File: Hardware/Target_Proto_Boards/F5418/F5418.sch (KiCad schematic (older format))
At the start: 51 parts, among them J1 LED_P4.1, J10 PORT4, J11 PORT8, J12 JTAG/SBW, J13 VCC, J14 GND, J15 +5V, J16 GND, J17 VSEL, J18 LogAna, J19 AS, J2 PORT1, J3 PORT5, J4 DEBUG, J5 PORT2, J6 PORT6, J7 USB_B_Micro, J8 PORT3, J9 PORT7, SW1 RESET, SW2 TL-2203, U1 MSP430F5418IPNR, U2 HT7533-1, Y1 32768 12pF, Y2 25 MHz

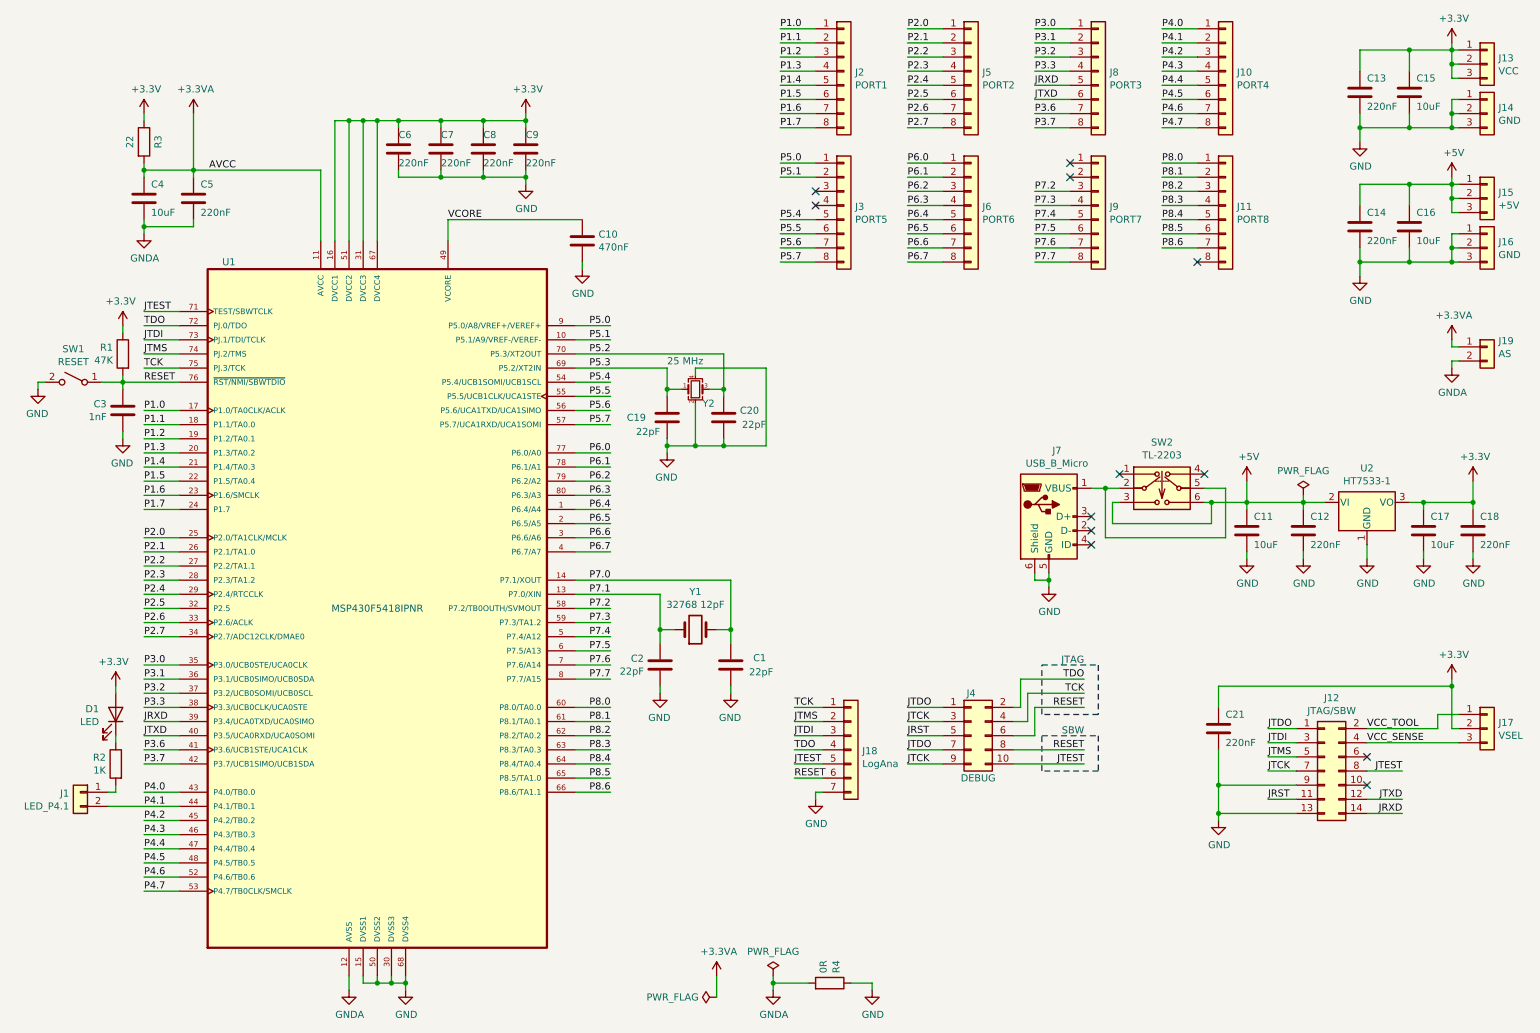
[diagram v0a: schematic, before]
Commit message: Updated Hardware Schematics and Boards
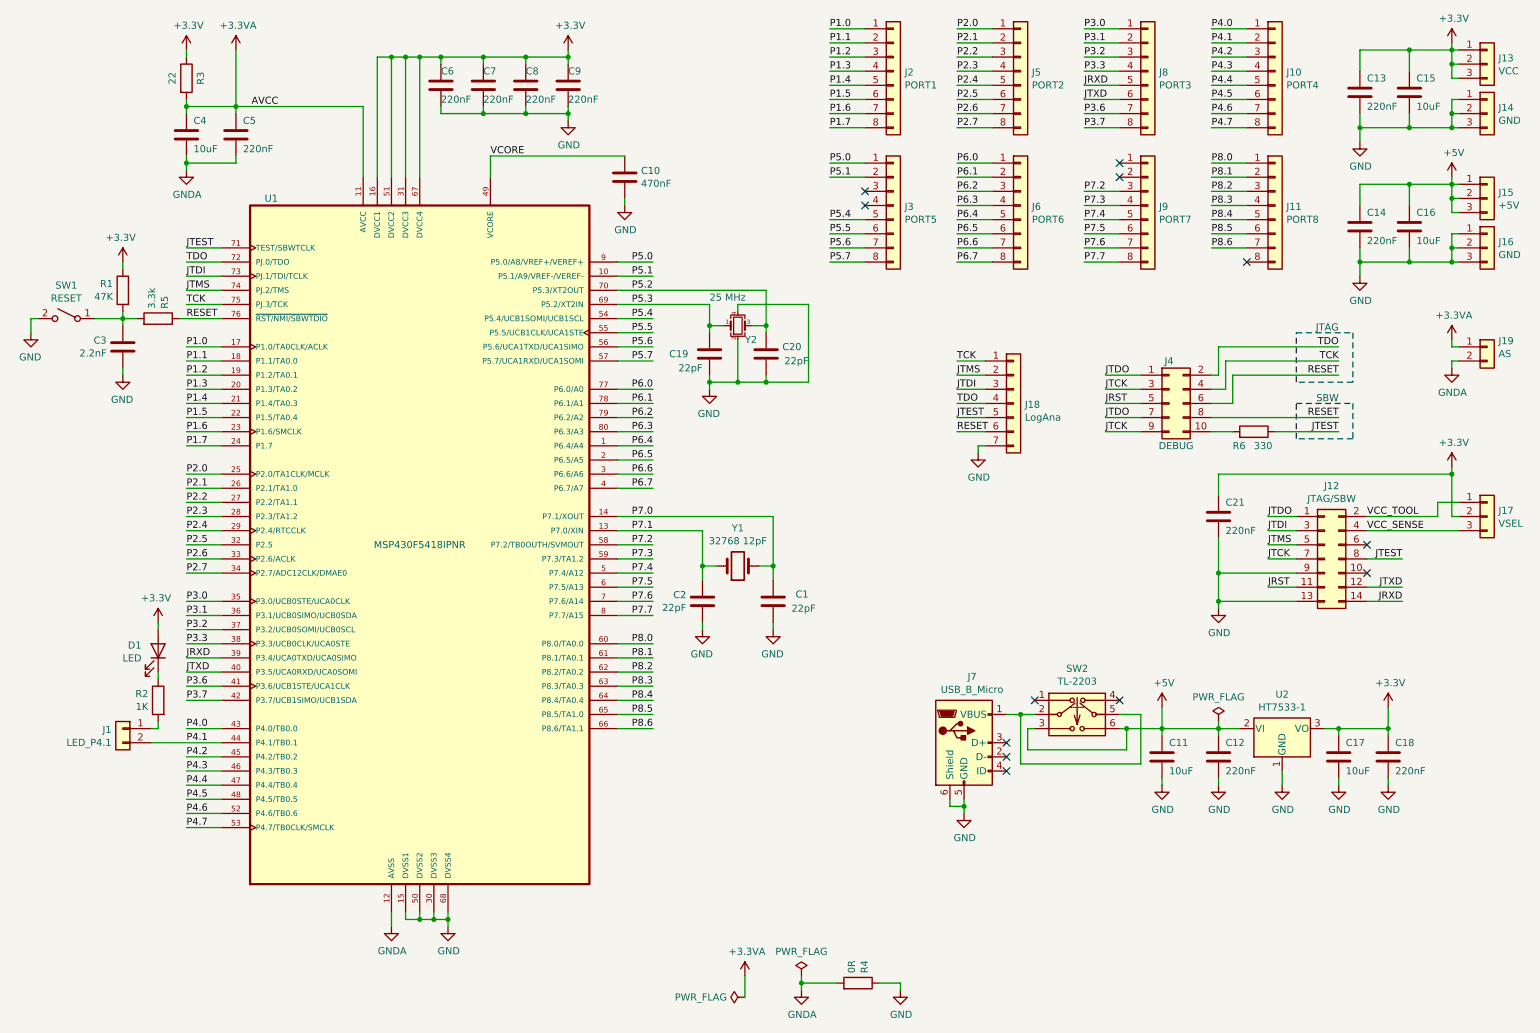
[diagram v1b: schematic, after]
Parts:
- added R5: 3.3k, Resistor_SMD:R_0603_1608Metric_Pad0.98x0.95mm_HandSolder, symbol Device:R
- added R6: 330, Resistor_SMD:R_0603_1608Metric_Pad0.98x0.95mm_HandSolder, symbol Device:R
- C3: value 1nF -> 2.2nF; Descr 0603 Multilayer Ceramic Capacitors MLCC - SMD/SMT ROHS -> X7R 2.2nF ±10% 50V 0603 Multilayer Ceramic Capacitors MLCC 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; LCSC C1588 -> C1604
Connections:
- net JTEST: now also R6.1; no longer J4.10 (Pin_10)
- net RESET: now also R5.1; no longer C3.1, R1.2, SW1.1 (A)
- new net: C3.1, R1.2, R5.2, SW1.1 (A)
- new net: J4.10 (Pin_10), R6.2
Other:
- moved on the sheet: C1, C10, C11, C12, C17, C18, C19, C2, C20, C21, C3, C4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
